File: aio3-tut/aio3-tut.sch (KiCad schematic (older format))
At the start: 20 parts, among them J1 USB_B, SW1 SW_Push, SW2 MX1, SW3 MX2, SW4 MX3, SW5 MX4, U1 ATmega32U4-AU, Y1 16MHz

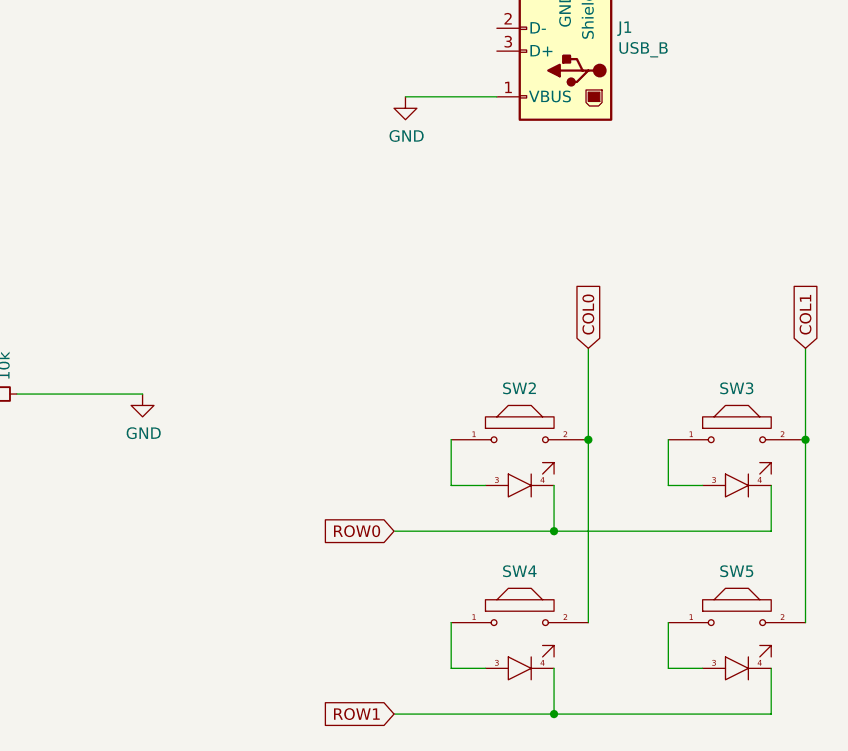
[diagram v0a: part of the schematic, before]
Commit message: fixes
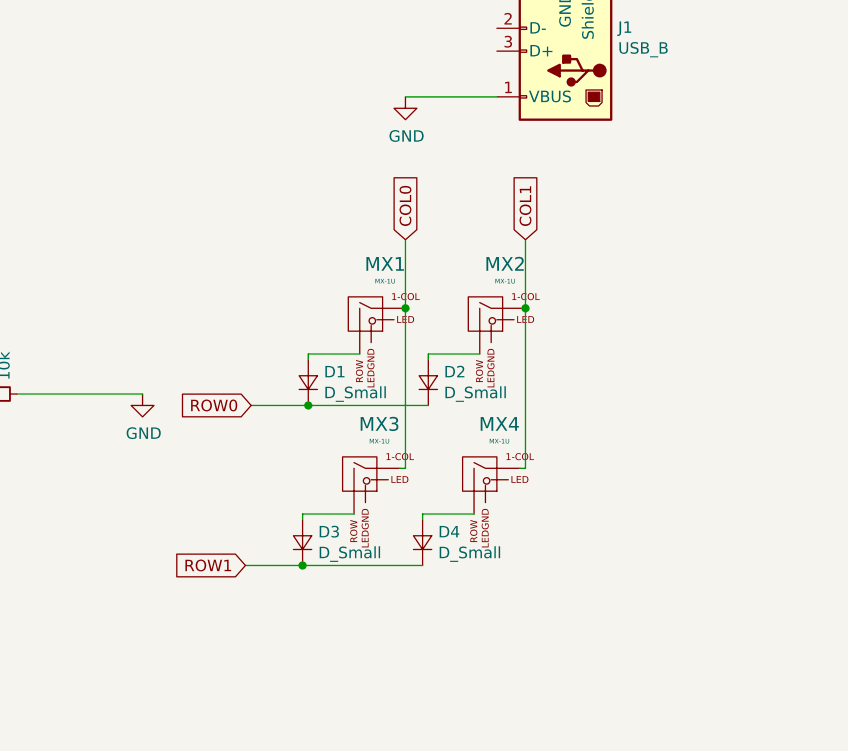
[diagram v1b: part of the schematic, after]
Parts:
- removed SW2: MX1, Keebio-Parts:MX-Alps-Choc-1U-NoLED, symbol keebio:MX
- removed SW3: MX2, Keebio-Parts:MX-Alps-Choc-1U-NoLED, symbol keebio:MX
- removed SW4: MX3, Keebio-Parts:MX-Alps-Choc-1U-NoLED, symbol keebio:MX
- removed SW5: MX4, Keebio-Parts:MX-Alps-Choc-1U-NoLED, symbol keebio:MX
- added D1, D2, D3, D4: D_Small, Diode_SMD:D_SOD-123, symbol Device:D_Small
- added MX1, MX2, MX3, MX4: MX-1U, MX_Alps_Hybrid:MX-1U, symbol MX_Alps_Hybrids:MX-1U
- U1: footprint Keebio-Parts:ArduinoProMicro-Mini-USB -> Housings_QFP:TQFP-44_10x10mm_Pitch0.8mm
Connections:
- wire segments 66 -> 64
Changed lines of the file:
@@
 F 0 "U1" H 3150 1011 50  0000 C CNN
 F 1 "ATmega32U4-AU" H 3150 920 50  0000 C CNN
-F 2 "Keebio-Parts:ArduinoProMicro-Mini-USB" H 3150 2900 50  0001 C CIN
+F 2 "Housings_QFP:TQFP-44_10x10mm_Pitch0.8mm" H 3150 2900 50  0001 C CIN
 F 3 "http://ww1.microchip.com/downloads/en/DeviceDoc/Atmel-7766-8-bit-AVR-ATmega16U4-32U4_Datasheet.pdf" H 3150 2900 50  0001 C CNN
 	1    3150 2900
@@
 	6400 2150 6000 2150
 $Comp
-L keebio:MX SW2
-U 1 1 5CC78594
-P 6500 3650
-F 0 "SW2" H 6500 3873 50  0000 C CNN
-F 1 "MX1" H 6500 3350 60  0001 C CNN
-F 2 "Keebio-Parts:MX-Alps-Choc-1U-NoLED" H 6500 3650 60  0001 C CNN
-F 3 "" H 6500 3650 60  0001 C CNN
-	1    6500 3650
-	1    0    0    -1
-$EndComp
-$Comp
-L keebio:MX SW3
-U 1 1 5CC794F6
-P 7450 3650
-F 0 "SW3" H 7450 3873 50  0000 C CNN
-F 1 "MX2" H 7450 3350 60  0001 C CNN
-F 2 "Keebio-Parts:MX-Alps-Choc-1U-NoLED" H 7450 3650 60  0001 C CNN
-F 3 "" H 7450 3650 60  0001 C CNN
-	1    7450 3650
-	1    0    0    -1
-$EndComp
-$Comp
-L keebio:MX SW4
-U 1 1 5CC7A134
-P 6500 4450
-F 0 "SW4" H 6500 4673 50  0000 C CNN
-F 1 "MX3" H 6500 4150 60  0001 C CNN
-F 2 "Keebio-Parts:MX-Alps-Choc-1U-NoLED" H 6500 4450 60  0001 C CNN
-F 3 "" H 6500 4450 60  0001 C CNN
-	1    6500 4450
-	1    0    0    -1
-$EndComp
-$Comp
-L keebio:MX SW5
-U 1 1 5CC7A756
-P 7450 4450
-F 0 "SW5" H 7450 4673 50  0000 C CNN
-F 1 "MX4" H 7450 4150 60  0001 C CNN
-F 2 "Keebio-Parts:MX-Alps-Choc-1U-NoLED" H 7450 4450 60  0001 C CNN
-F 3 "" H 7450 4450 60  0001 C CNN
-	1    7450 4450
-	1    0    0    -1
-$EndComp
-Wire Wire Line
-	7600 4650 7600 4850
-Wire Wire Line
-	7600 4850 6650 4850
-Wire Wire Line
-	6650 4850 6650 4650
-Wire Wire Line
-	6650 4850 5950 4850
-Connection ~ 6650 4850
-Wire Wire Line
-	7600 3850 7600 4050
-Wire Wire Line
-	7600 4050 6650 4050
-Wire Wire Line
-	6650 4050 6650 3850
-Wire Wire Line
-	6650 4050 5950 4050
-Connection ~ 6650 4050
-Wire Wire Line
-	7150 4450 7150 4650
-Wire Wire Line
-	7150 4650 7300 4650
-Wire Wire Line
-	6350 4650 6200 4650
-Wire Wire Line
-	6200 4650 6200 4450
-Wire Wire Line
-	6350 3850 6200 3850
-Wire Wire Line
-	6200 3850 6200 3650
-Wire Wire Line
-	7300 3850 7150 3850
-Wire Wire Line
-	7150 3850 7150 3650
-Wire Wire Line
-	6800 3650 6800 4450
-Wire Wire Line
-	7750 4450 7750 3650
-Wire Wire Line
-	7750 3650 7750 3250
-Connection ~ 7750 3650
-Wire Wire Line
-	6800 3650 6800 3250
-Connection ~ 6800 3650
-Text GLabel 5950 4050 0    50   Input ~ 0
+L MX_Alps_Hybrids:MX-1U MX1
+U 1 1 5CBFD9AE
+P 5825 3100
+F 0 "MX1" H 5911 3317 60  0000 C CNN
+F 1 "MX-1U" H 5911 3243 20  0000 C CNN
+F 2 "MX_Alps_Hybrid:MX-1U" H 5800 3075 60  0001 C CNN
+F 3 "" H 5800 3075 60  0001 C CNN
+	1    5825 3100
+	1    0    0    -1
+$EndComp
+Wire Wire Line
+	5800 3275 5575 3275
+Wire Wire Line
+	5575 3275 5575 3300
+$Comp
+L Device:D_Small D1
+U 1 1 5CBFFA52
+P 5575 3400
+F 0 "D1" V 5621 3332 50  0000 R CNN
+F 1 "D_Small" V 5530 3332 50  0000 R CNN
+F 2 "Diode_SMD:D_SOD-123" V 5575 3400 50  0001 C CNN
+F 3 "~" V 5575 3400 50  0001 C CNN
+	1    5575 3400
+	0    -1   -1   0
+$EndComp
+$Comp
+L MX_Alps_Hybrids:MX-1U MX2
+U 1 1 5CC15172
+P 6350 3100
+F 0 "MX2" H 6436 3317 60  0000 C CNN
+F 1 "MX-1U" H 6436 3243 20  0000 C CNN
+F 2 "MX_Alps_Hybrid:MX-1U" H 6325 3075 60  0001 C CNN
+F 3 "" H 6325 3075 60  0001 C CNN
+	1    6350 3100
+	1    0    0    -1
+$EndComp
+Wire Wire Line
+	6325 3275 6100 3275
+Wire Wire Line
+	6100 3275 6100 3300
+$Comp
+L Device:D_Small D2
+U 1 1 5CC1517E
+P 6100 3400
+F 0 "D2" V 6146 3332 50  0000 R CNN
+F 1 "D_Small" V 6055 3332 50  0000 R CNN
+F 2 "Diode_SMD:D_SOD-123" V 6100 3400 50  0001 C CNN
+F 3 "~" V 6100 3400 50  0001 C CNN
+	1    6100 3400
+	0    -1   -1   0
+$EndComp
+Wire Wire Line
+	5775 3975 5550 3975
+Wire Wire Line
+	5550 3975 5550 4000
+$Comp
+L Device:D_Small D3
+U 1 1 5CC192AE
+P 5550 4100
+F 0 "D3" V 5596 4032 50  0000 R CNN
+F 1 "D_Small" V 5505 4032 50  0000 R CNN
+F 2 "Diode_SMD:D_SOD-123" V 5550 4100 50  0001 C CNN
+F 3 "~" V 5550 4100 50  0001 C CNN
+	1    5550 4100
+	0    -1   -1   0
+$EndComp
+$Comp
+L MX_Alps_Hybrids:MX-1U MX4
+U 1 1 5CC192B8
+P 6325 3800
+F 0 "MX4" H 6411 4017 60  0000 C CNN
+F 1 "MX-1U" H 6411 3943 20  0000 C CNN
+F 2 "MX_Alps_Hybrid:MX-1U" H 6300 3775 60  0001 C CNN
+F 3 "" H 6300 3775 60  0001 C CNN
+	1    6325 3800
+	1    0    0    -1
+$EndComp
+Wire Wire Line
+	6300 3975 6075 3975
+Wire Wire Line
+	6075 3975 6075 4000
+$Comp
+L Device:D_Small D4
+U 1 1 5CC192C4
+P 6075 4100
+F 0 "D4" V 6121 4032 50  0000 R CNN
+F 1 "D_Small" V 6030 4032 50  0000 R CNN
+F 2 "Diode_SMD:D_SOD-123" V 6075 4100 50  0001 C CNN
+F 3 "~" V 6075 4100 50  0001 C CNN
+	1    6075 4100
+	0    -1   -1   0
+$EndComp
+Wire Wire Line
+	6000 3075 6000 3775
+Wire Wire Line
+	6000 3775 5975 3775
+$Comp
+L MX_Alps_Hybrids:MX-1U MX3
+U 1 1 5CC192A2
+P 5800 3800
+F 0 "MX3" H 5886 4017 60  0000 C CNN
+F 1 "MX-1U" H 5886 3943 20  0000 C CNN
+F 2 "MX_Alps_Hybrid:MX-1U" H 5775 3775 60  0001 C CNN
+F 3 "" H 5775 3775 60  0001 C CNN
+	1    5800 3800
+	1    0    0    -1
+$EndComp
+Wire Wire Line
+	6525 3075 6525 3775
+Wire Wire Line
+	6525 3775 6500 3775
+Wire Wire Line
+	6075 4200 5550 4200
+Wire Wire Line
+	6100 3500 5575 3500
+Wire Wire Line
+	6000 3075 6000 2775
+Connection ~ 6000 3075
+Wire Wire Line
+	6525 3075 6525 2775
+Connection ~ 6525 3075
+Wire Wire Line
+	5550 4200 5300 4200
+Connection ~ 5550 4200
+Connection ~ 5575 3500
+Wire Wire Line
+	5575 3500 5325 3500
+Text GLabel 5325 3500 0    50   Input ~ 0
 ROW0
-Text GLabel 5950 4850 0    50   Input ~ 0
+Text GLabel 5300 4200 0    50   Input ~ 0
 ROW1
-Text GLabel 6800 3250 1    50   Input ~ 0
+Text GLabel 6000 2775 1    50   Input ~ 0
 COL0
-Text GLabel 7750 3250 1    50   Input ~ 0
+Text GLabel 6525 2775 1    50   Input ~ 0
 COL1
 $EndSCHEMATC
